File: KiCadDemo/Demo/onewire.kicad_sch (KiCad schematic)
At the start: 5 parts, among them J2 22-05-7025, M1 BSS84, U4 DS1822-PAR

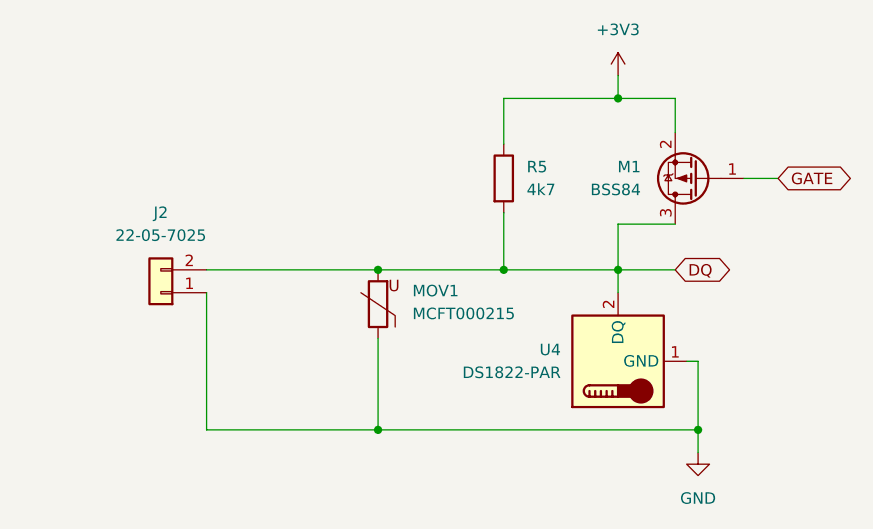
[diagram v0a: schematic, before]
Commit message: Add files via upload
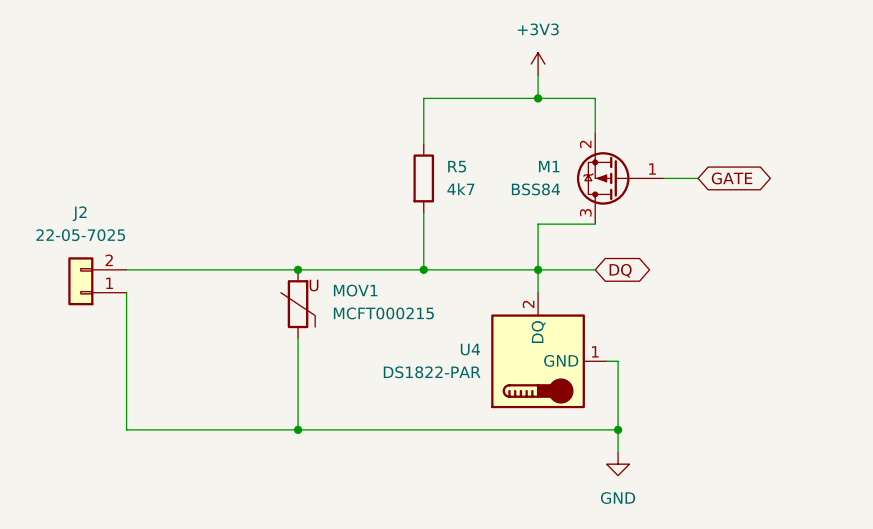
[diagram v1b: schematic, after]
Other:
- moved on the sheet: J2, M1, MOV1, R5, U4

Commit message: Check #4
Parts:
- J2: footprint (none) -> Demo:IO2
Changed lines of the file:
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@@
       (effects (font (size 1.27 1.27)))
     )
-    (property "Footprint" "" (at 110.49 93.98 0)
+    (property "Footprint" "Demo:IO2" (at 110.49 93.98 0)
       (effects (font (size 1.27 1.27)) hide)
     )
